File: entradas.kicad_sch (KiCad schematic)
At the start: 16 parts, among them J4 entrada discreta, J5 entrada discreta, SW1 SW_MEC_5E, SW2 SW_MEC_5E, U4 LTV-817-C, U5 LTV-817-C

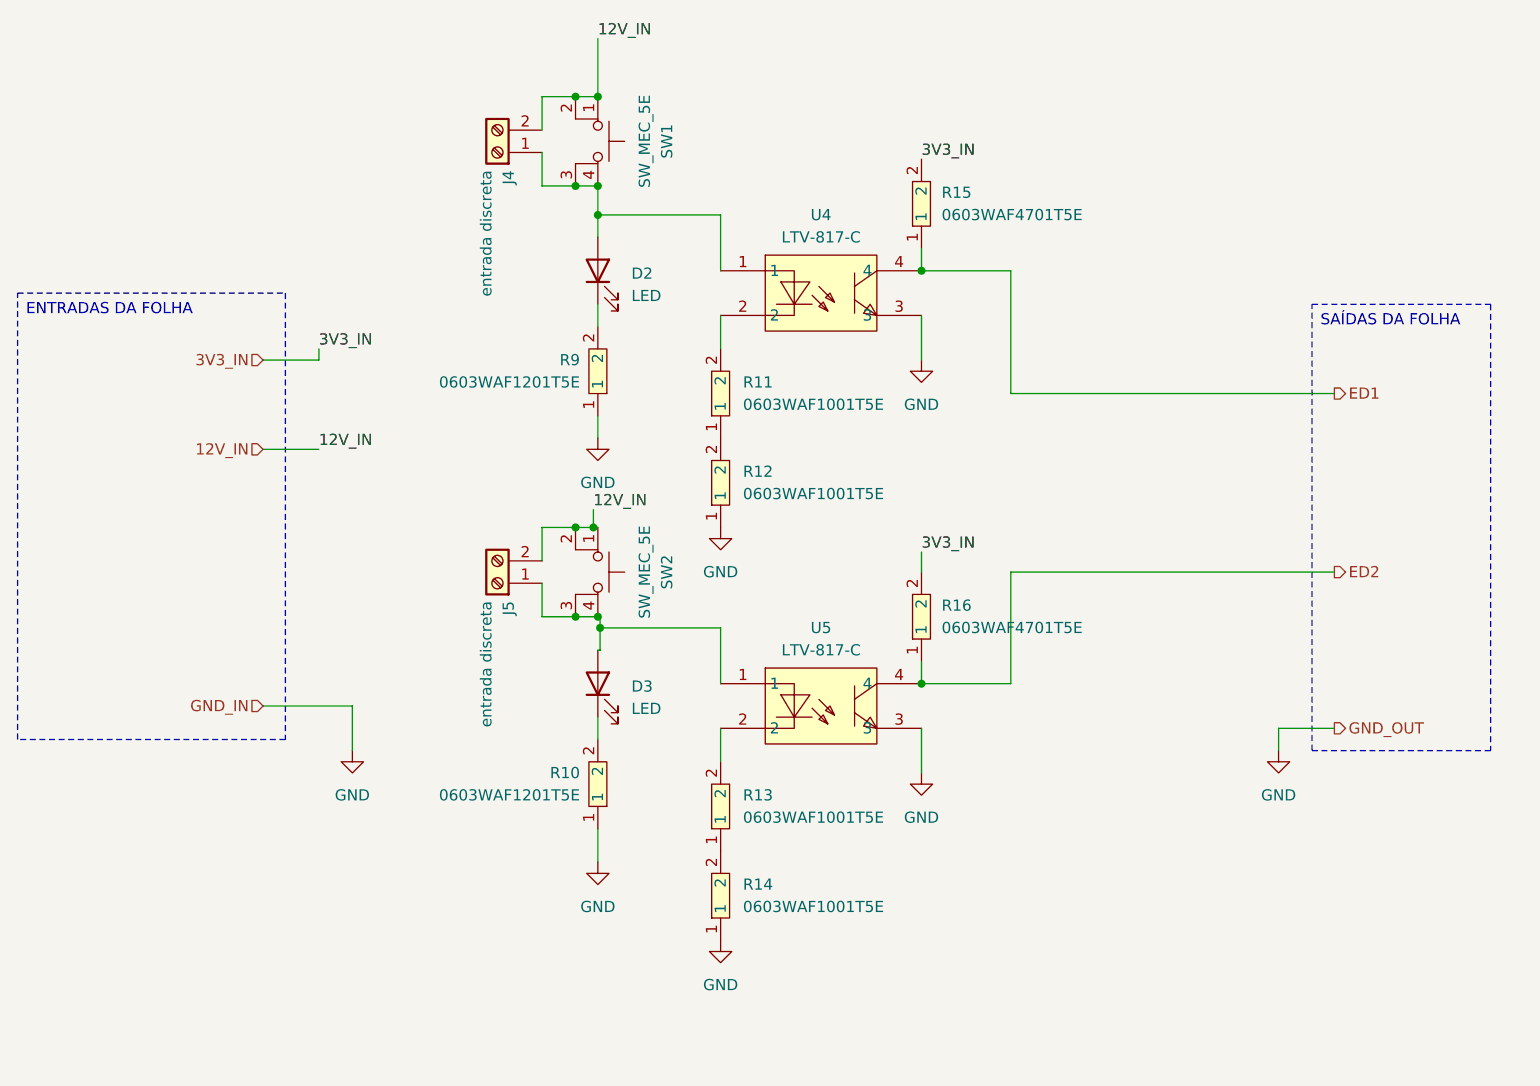
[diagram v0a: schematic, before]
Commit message: organização e legendas do esquemático
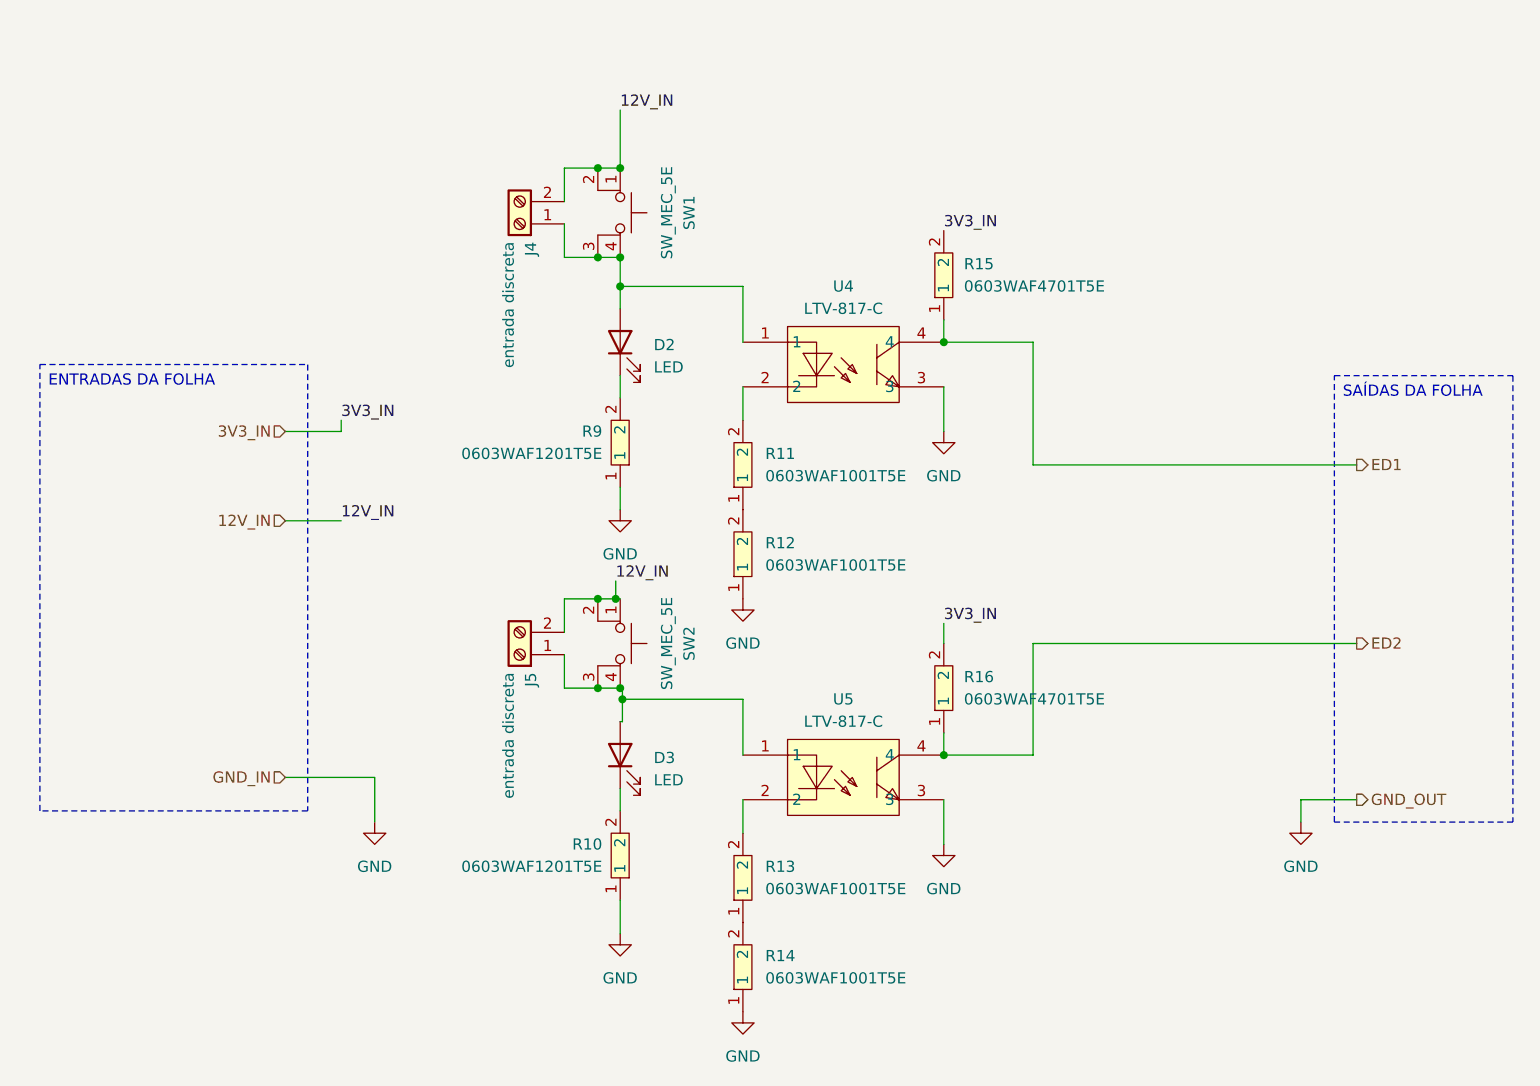
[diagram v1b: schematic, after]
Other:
- moved on the sheet: D2, D3, J4, J5, R10, R11, R12, R13, R14, R15, R16, R9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
